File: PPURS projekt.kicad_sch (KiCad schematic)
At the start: 26 parts, among them J2 AVR-ISP-10, J3 Barrel_Jack, SW1 SW_Push_Dual, SW2 SW_Push_Dual, U1 ATmega16A-P, U2 004-0-0053, U3 LM35-LP, U4 LCD-016N002L, Y1 8Mhz

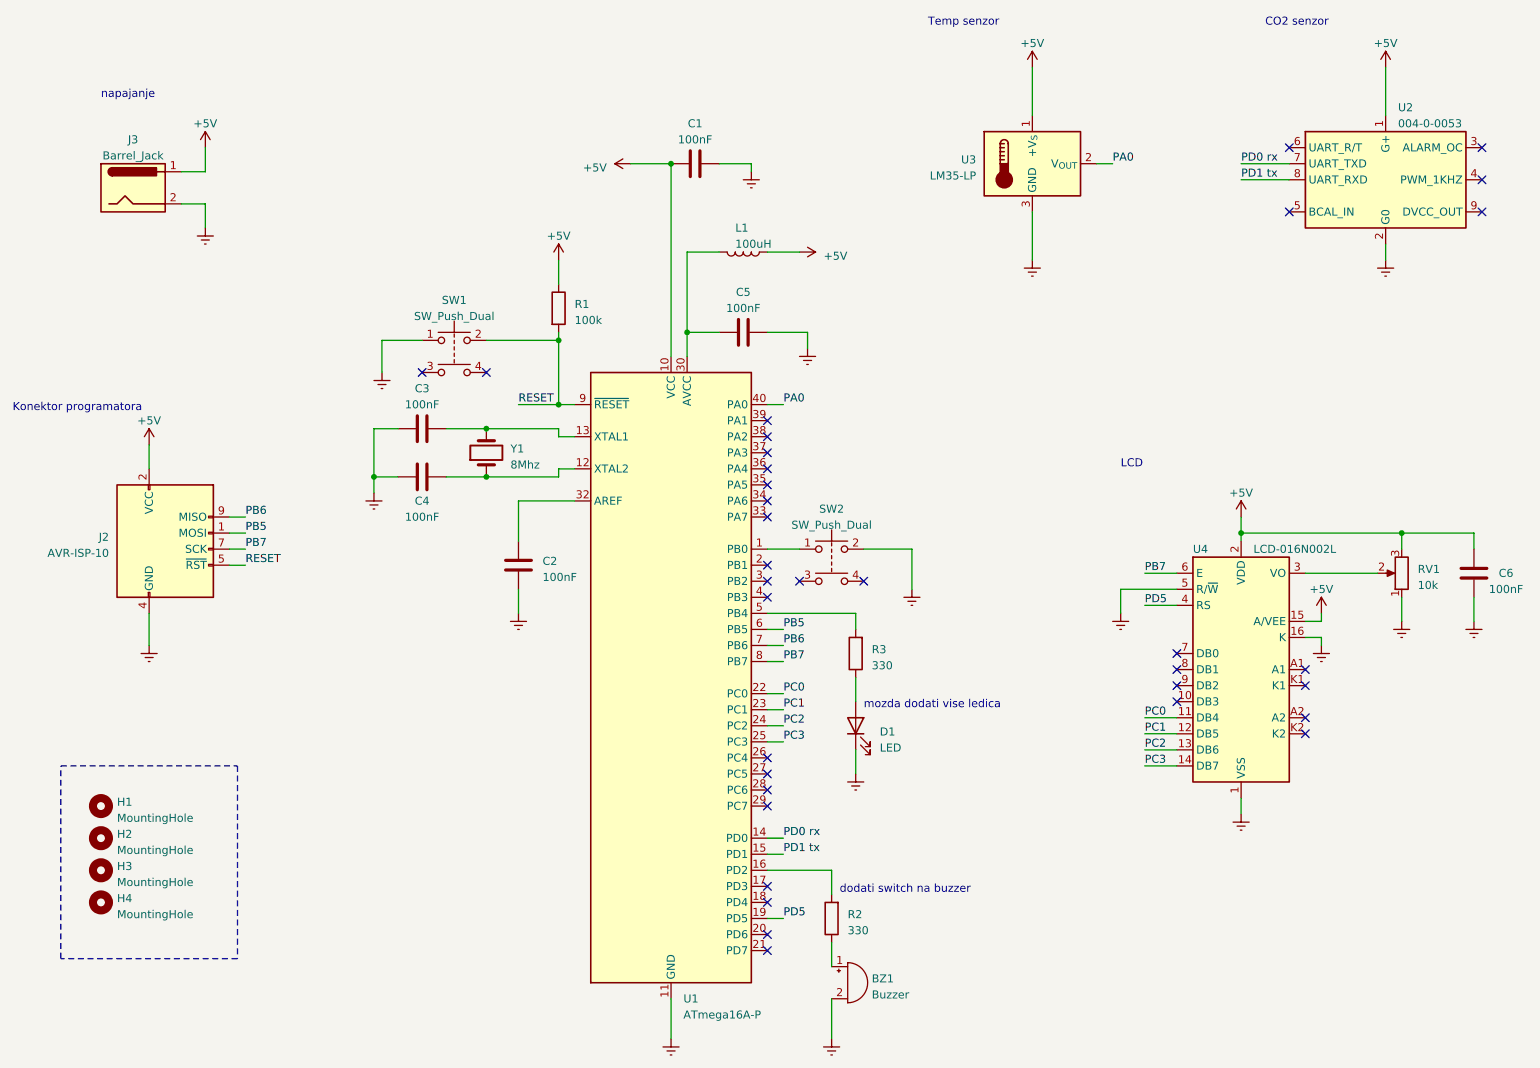
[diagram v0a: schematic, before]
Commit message: Add files via upload
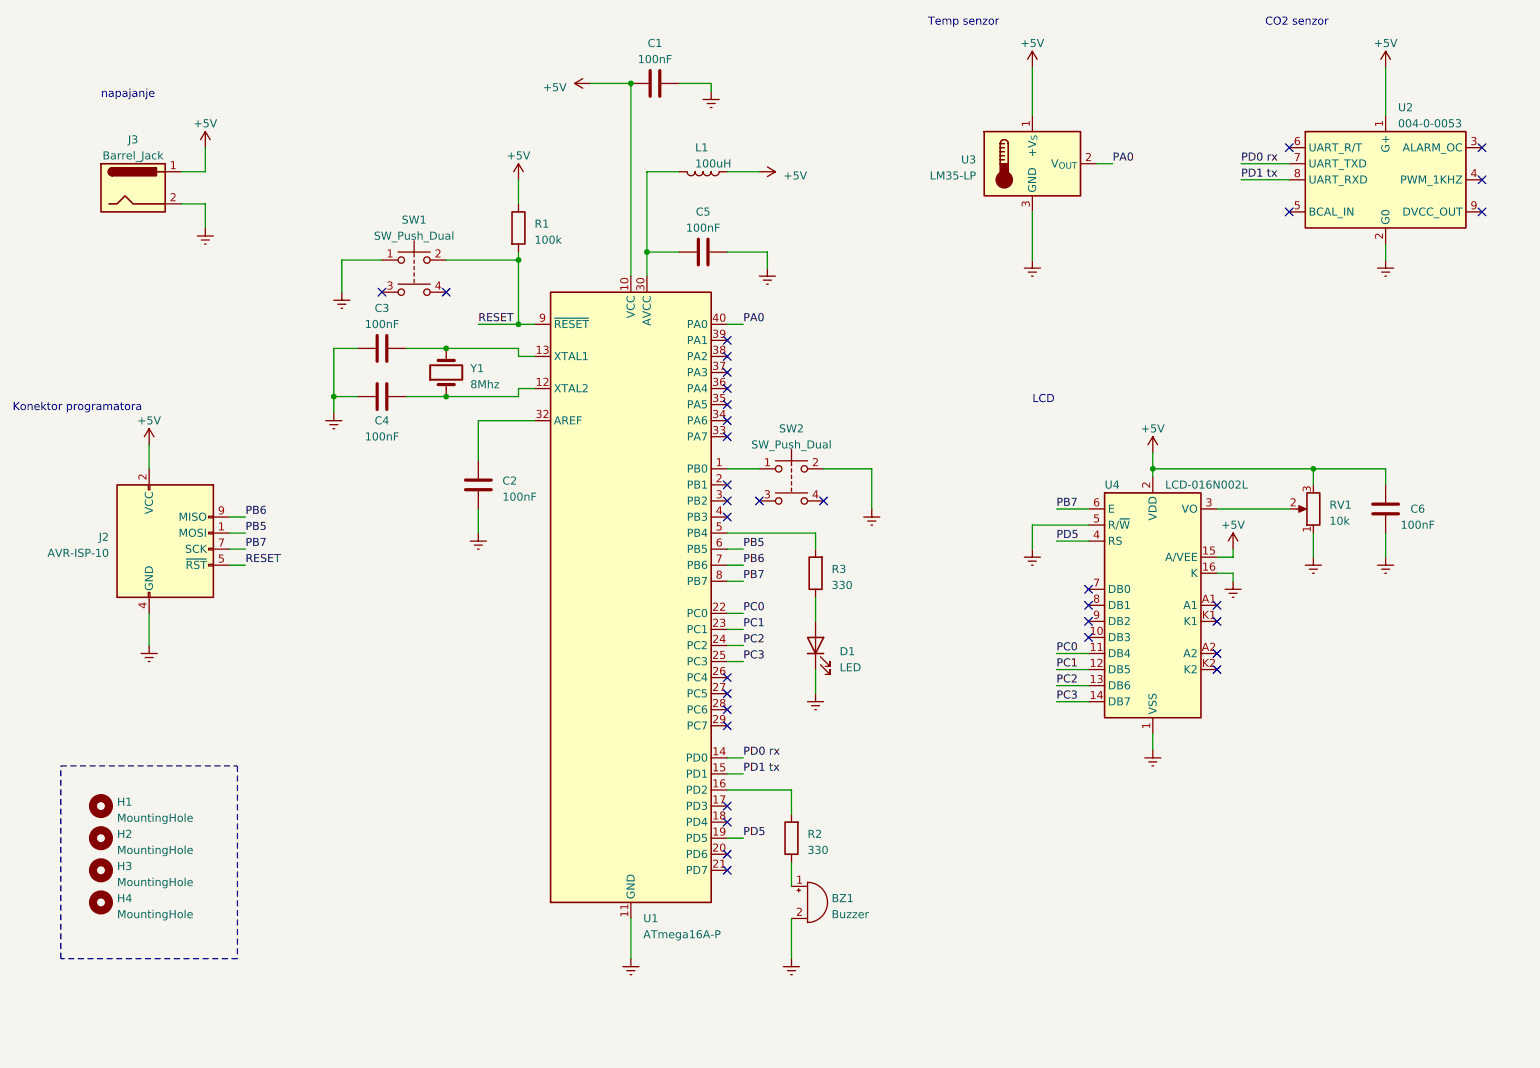
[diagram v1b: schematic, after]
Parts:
- C1, C2, C3, C4, C5, C6: footprint Library:CP_Radial_Tantal_D5.0mm_P5.00mmjm -> Library:CP_Radial_Tantal_D5.0mm_P5.00mmJM
- D1: footprint LED_THT:LED_D3.0mm_FlatTop -> LED_THT:LED_D5.0mm_Clear
- J3: footprint Library:BarrelJack_CUI_PJ-063AH_Horizontaljm -> Library:BarrelJack_CUI_PJ-063AH_HorizontalJM
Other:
- note removed: "dodati switch na buzzer"
- note removed: "mozda dodati vise ledica"
- title: (none) -> CO2 alarm sa ATmega16A-P
- moved on the sheet: BZ1, C1, C2, C3, C4, C5, C6, D1, L1, R1, R2, R3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
